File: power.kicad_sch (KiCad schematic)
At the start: 10 parts, among them J9 Barrel_Jack_Switch, U8 L7805, U9 AMS1117CD-3.3

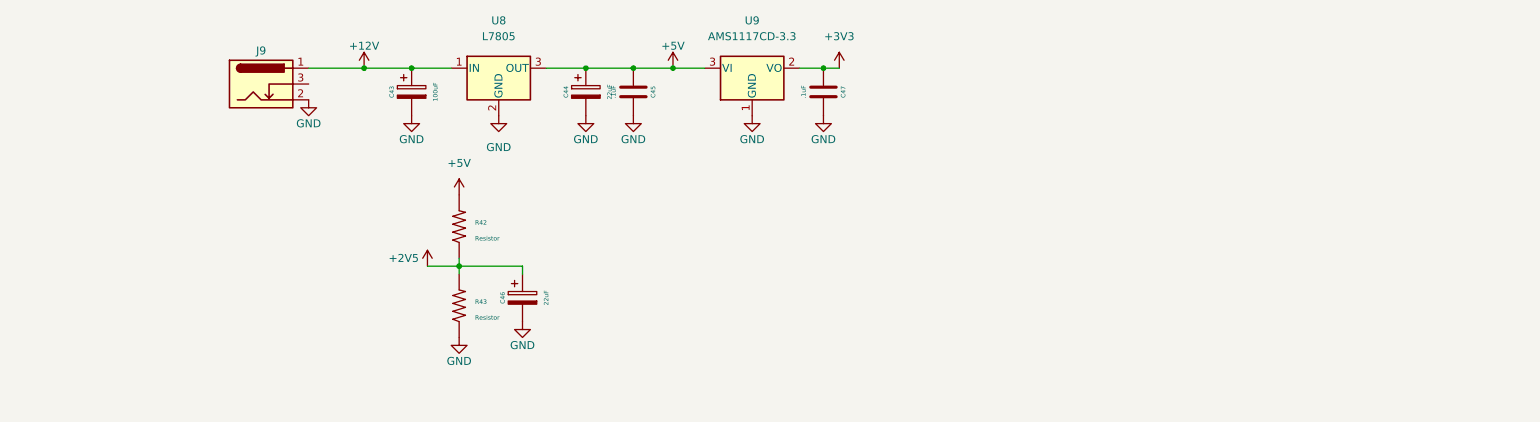
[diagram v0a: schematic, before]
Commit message: Add files via upload
Added "WIP" branch, which is some of my mods.
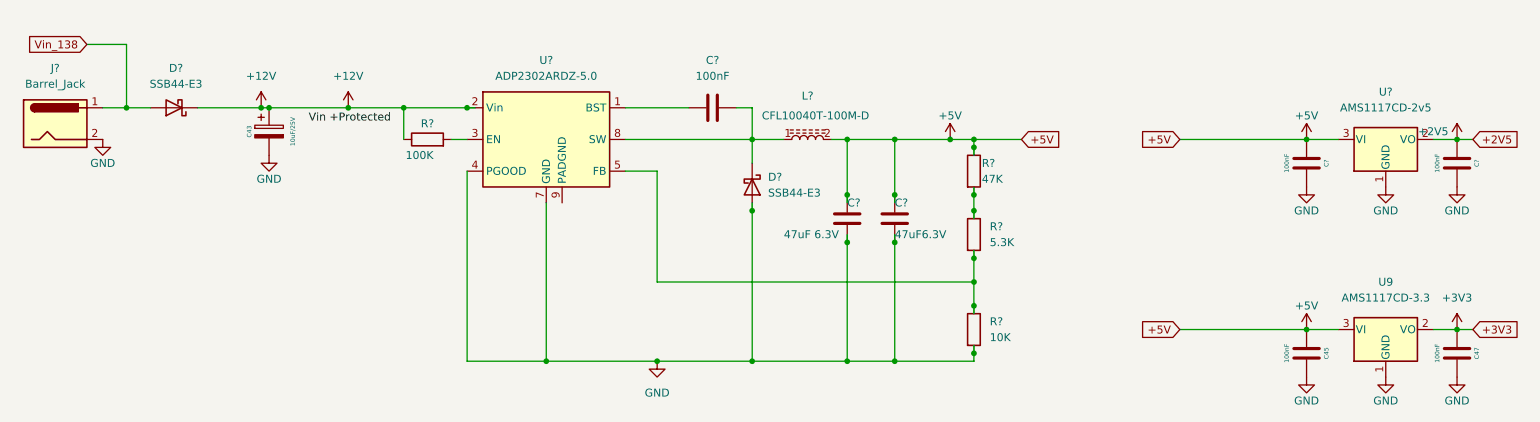
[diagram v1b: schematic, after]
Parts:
- removed C44, C46: 22uF, Capacitor_SMD:CP_Elec_4x5.4, symbol Xenir:Cap_Polarized
- removed J9: Barrel_Jack_Switch, Xenir:BarrelJack_Horizontal, symbol Connector:Barrel_Jack_Switch
- removed R42, R43: Resistor, Resistor_SMD:R_0805_2012Metric, symbol Xenir:Resistor
- removed U8: L7805, Package_TO_SOT_SMD:TO-252-3_TabPin2, symbol Regulator_Linear:L7805
- added C?: 100nF, Capacitor_SMD:C_0805_2012Metric_Pad1.18x1.45mm_HandSolder, symbol Device:C
- added C? (x2): 100nF, Capacitor_SMD:C_0805_2012Metric_Pad1.18x1.45mm_HandSolder, symbol Xenir:Capacitor
- added C?: 47uF 6.3V, Capacitor_SMD:C_0805_2012Metric_Pad1.18x1.45mm_HandSolder, symbol Device:C
- added C?: 47uF6.3V, Capacitor_SMD:C_0805_2012Metric_Pad1.18x1.45mm_HandSolder, symbol Device:C
- added D?: SSB44-E3, symbol Device:D_Schottky
- added D?: SSB44-E3, Diode_SMD:D_SMA-SMB_Universal_Handsoldering, symbol Device:D_Schottky
- added J?: Barrel_Jack, symbol Connector:Barrel_Jack
- added L?: CFL10040T-100M-D, symbol Device:CFL10040T-100M-D
- added R?: 5.3K, symbol Device:R
- added R?: 47K, Resistor_SMD:R_0805_2012Metric_Pad1.20x1.40mm_HandSolder, symbol Device:R
- added R?: 10K, symbol Device:R
- added R?: 100K, Resistor_SMD:R_0805_2012Metric_Pad1.20x1.40mm_HandSolder, symbol Device:R
- added U?: ADP2302ARDZ-5.0, Package_SO:SOIC-8-1EP_3.9x4.9mm_P1.27mm_EP2.29x3mm, symbol Regulator_Switching:ADP2302ARDZ-5.0
- added U?: AMS1117CD-2v5, Package_TO_SOT_SMD:TO-252-3_TabPin2, symbol Regulator_Linear:AMS1117CD-3.3
- C43: value 100uF -> 10uF/25V; footprint Capacitor_SMD:CP_Elec_6.3x5.4 -> Capacitor_SMD:C_1206_3216Metric_Pad1.33x1.80mm_HandSolder
- C45, C47: value .1uF -> 100nF; footprint Xenir:Capacitor 0805 -> Capacitor_SMD:C_0805_2012Metric_Pad1.18x1.45mm_HandSolder
- U9: footprint Package_TO_SOT_SMD:SOT-223-3_TabPin2 -> Package_TO_SOT_SMD:TO-252-3_TabPin2
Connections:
- net +12V: now also D?.1 (K), R?.1, U?.2 (Vin)
- net +2V5: now also C?.1, U?.2 (VO)
- net +5V: now also C?.1, C?.1, C?.1, L?.2, R?.1, U?.3 (VI)
- net GND: now also C?.2, C?.2, C?.2, C?.2, D?.2 (A), J?.2, R?.2, U?.1 (GND), U?.4 (PGOOD), U?.7 (GND)
- new net: C?.2, D?.1 (K), L?.1, U?.8 (SW)
- new net: R?.1, R?.2
- new net: R?.1, R?.2, U?.5 (FB)
- new net: C?.1, U?.1 (BST)
- new net: R?.2, U?.3 (EN)
- new net Vin_138: D?.2 (A), J?.1
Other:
- moved on the sheet: C43, C45, C47, U9
